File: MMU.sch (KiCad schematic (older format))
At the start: 8 parts, among them U18 74LS08, U2 74LS138, U3 MMU

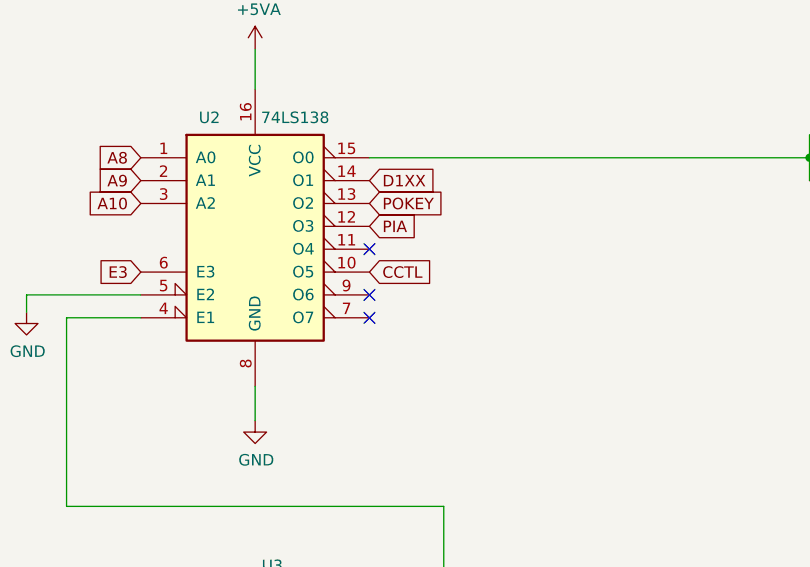
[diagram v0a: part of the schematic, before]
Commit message: Diagnostic
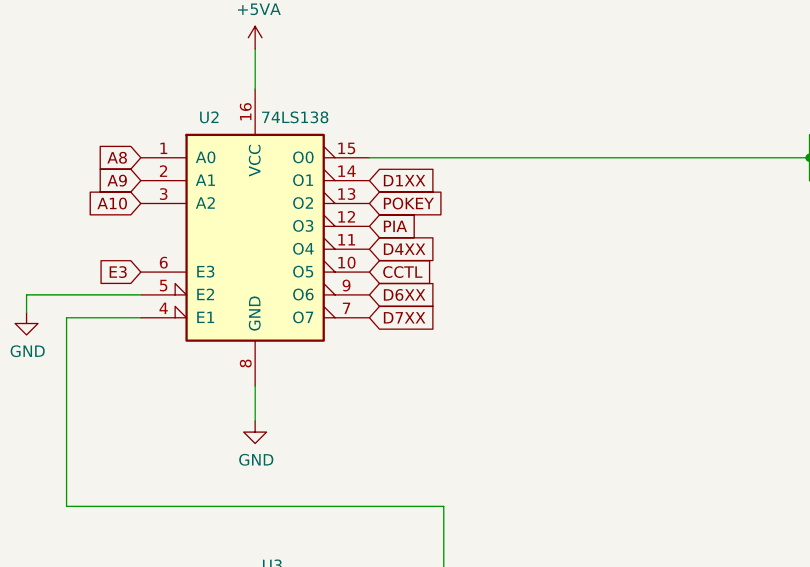
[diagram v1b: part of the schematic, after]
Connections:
- net D4XX: now reaches U2.11 (O4)
- net D7XX: now reaches U2.7 (O7)
- net D6XX: now reaches U2.9 (O6)
- no-connect marks 3 -> 0
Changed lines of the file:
@@
 Text GLabel 5875 2250 2    50   Input ~ 0
 POKEY
-NoConn ~ 5875 2450
-NoConn ~ 5875 2650
-NoConn ~ 5875 2750
 $Comp
 L 74xx:74LS08 U18
@@
 	1    0    0    -1
 $EndComp
+Text GLabel 5875 2650 2    50   Input ~ 0
+D6XX
+Text GLabel 5875 2450 2    50   Input ~ 0
+D4XX
+Text GLabel 5875 2750 2    50   Input ~ 0
+D7XX
 $EndSCHEMATC
